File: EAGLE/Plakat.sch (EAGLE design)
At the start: 25 parts, among them X1 USB-MICROB

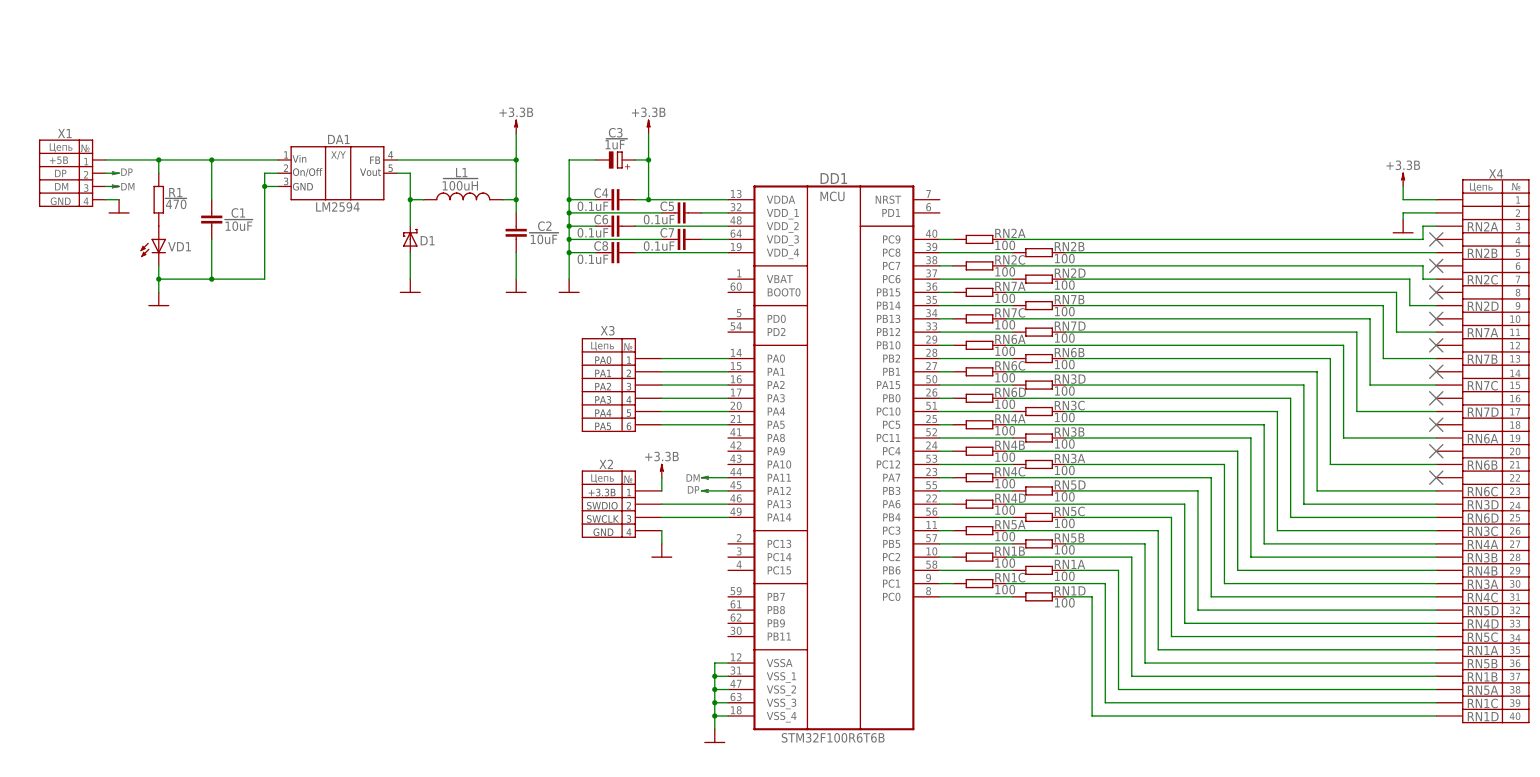
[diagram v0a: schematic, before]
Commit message: Modified СБ, Э3, ПП
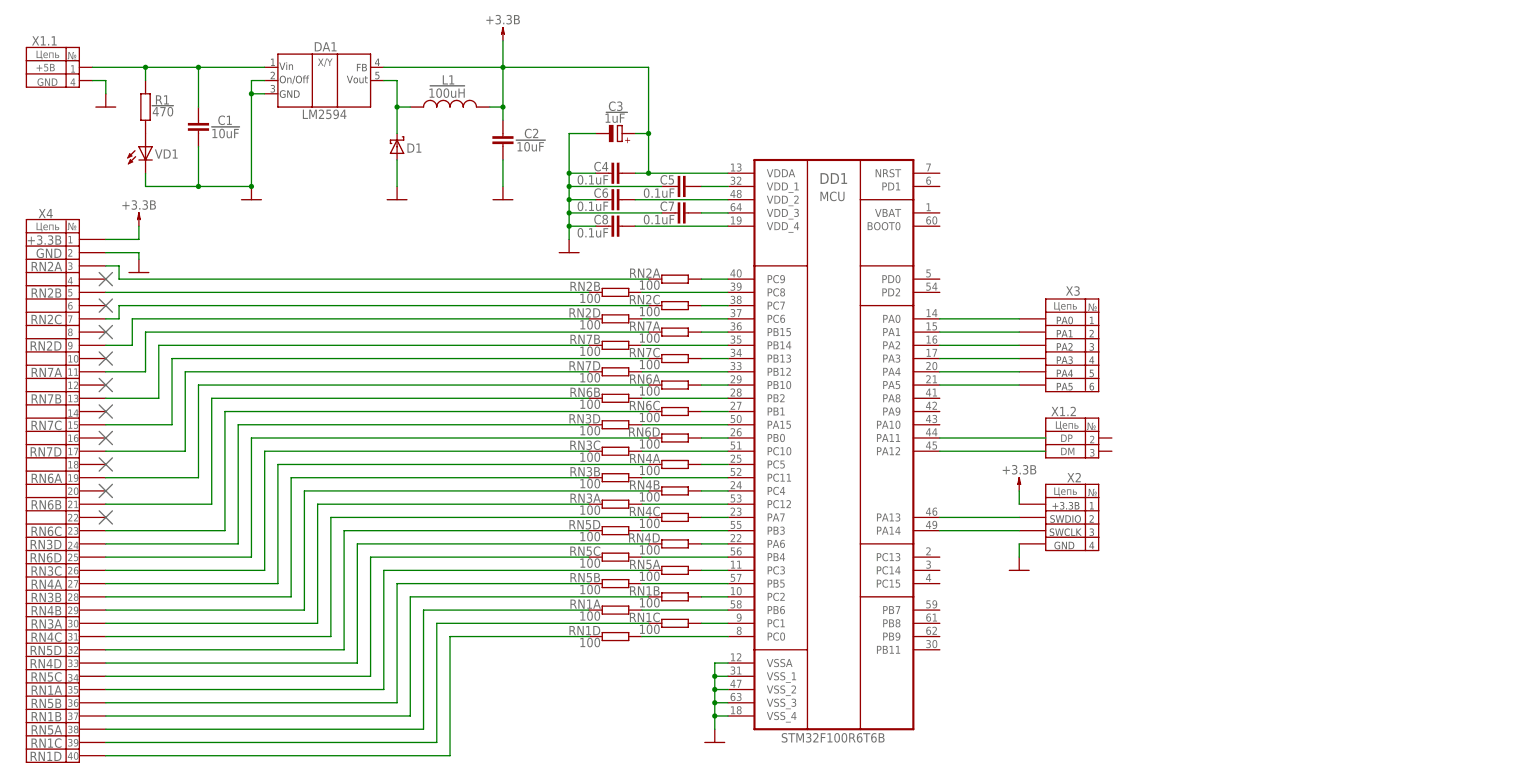
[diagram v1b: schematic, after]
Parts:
- removed X1: USB-MICROB, SparkFun-Connectors:USB-MICROB
- added X1.1, X1.2: (no value), pinhead:PINHD-1X2
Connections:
- removed net DM: DD1.PA11, X1.D-
- removed net DP: DD1.PA12, X1.D+
- new net N$67: DD1.PA11
- new net N$70: DD1.PA12
- net GND: now also X1.1.2; no longer X1.GND
- net N$1: now also X1.1.1; no longer X1.VBUS
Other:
- moved on the sheet: C1, C2, C3, C4, C5, C6, C7, C8, D1, DA1, DD1, L1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
